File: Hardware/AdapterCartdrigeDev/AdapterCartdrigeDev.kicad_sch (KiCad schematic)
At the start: 4 parts, among them J1 ROM, U1 28C256

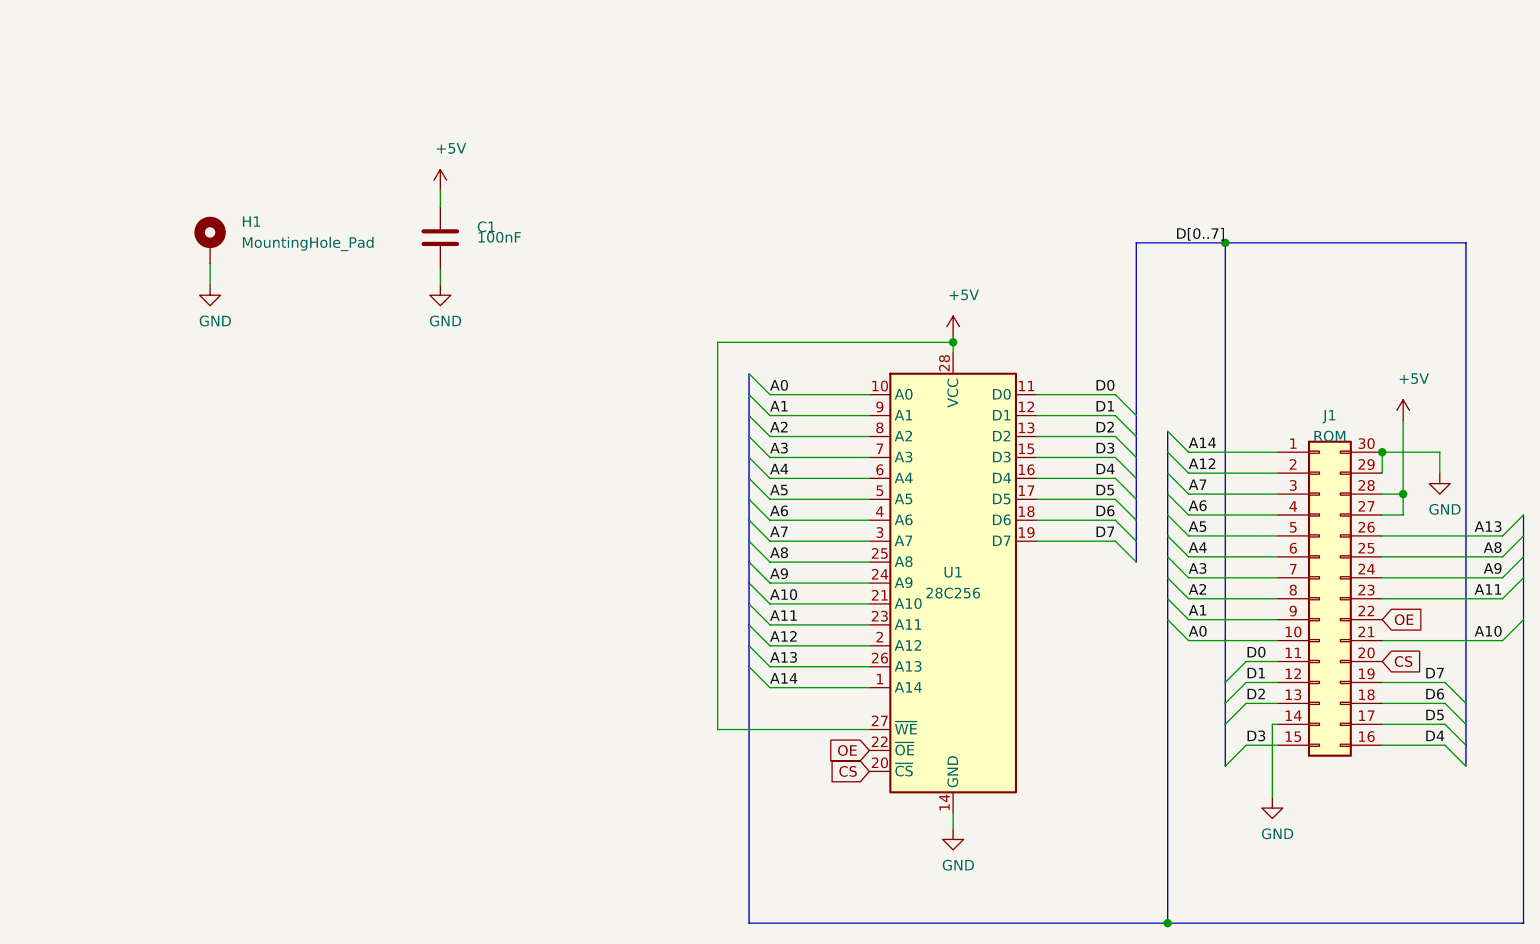
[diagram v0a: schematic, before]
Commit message: Fix
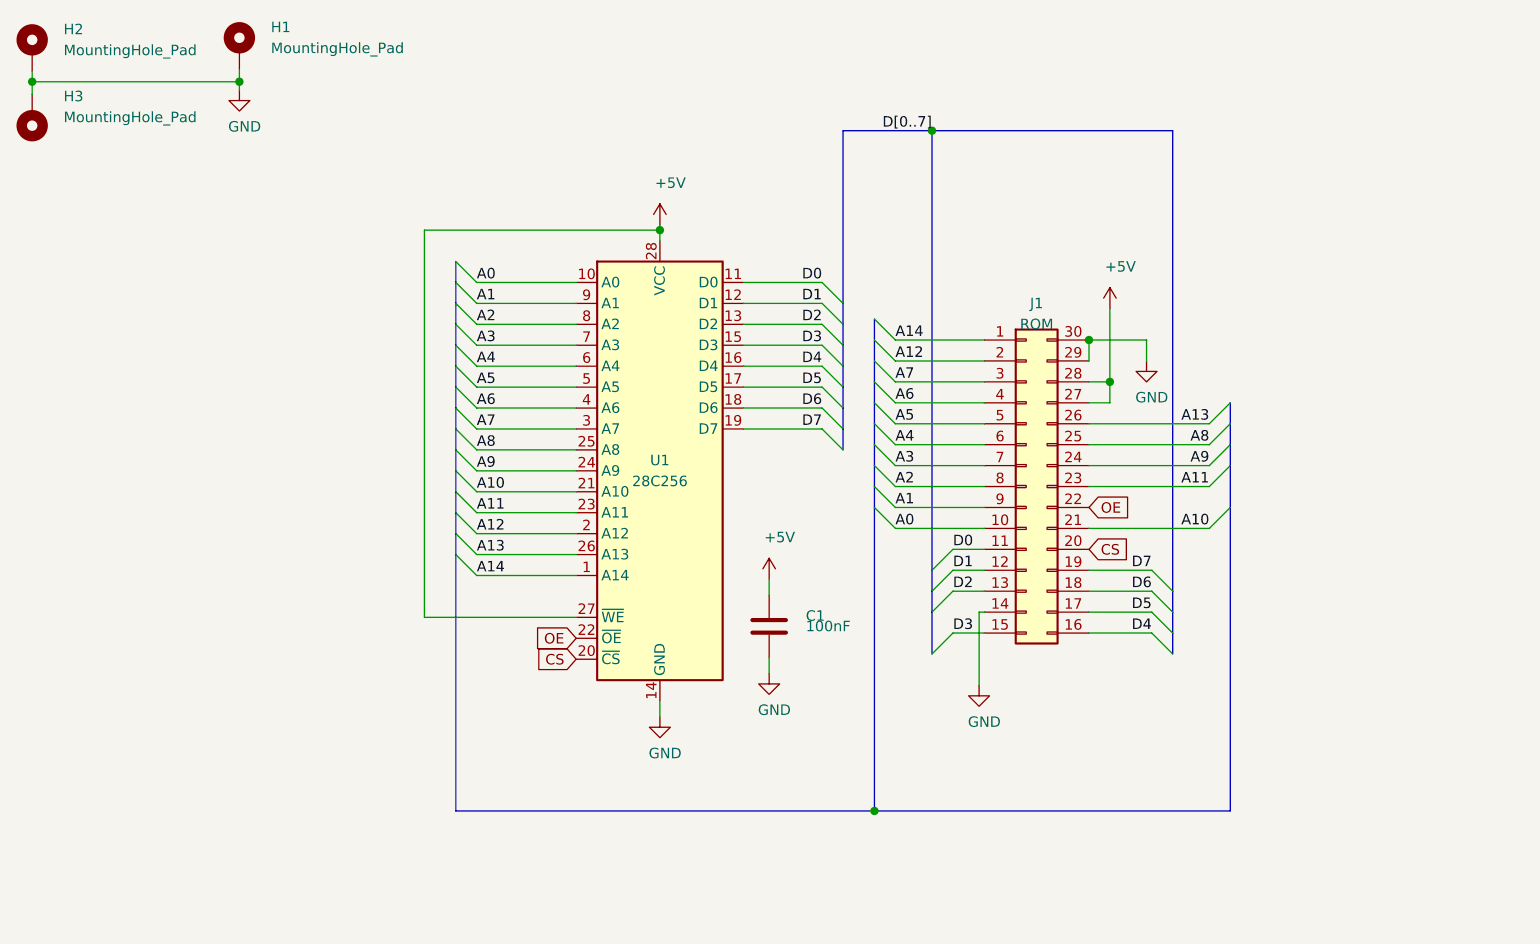
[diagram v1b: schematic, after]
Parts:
- added H2, H3: MountingHole_Pad, MountingHole:MountingHole_3.2mm_M3, symbol Mechanical:MountingHole_Pad
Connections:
- net GND: now also H2.1, H3.1
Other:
- moved on the sheet: C1, H1, J1, U1
